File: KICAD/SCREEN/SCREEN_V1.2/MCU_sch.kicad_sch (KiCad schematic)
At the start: 57 parts, among them SW6 SW_SPDT, SW9 SW_SPDT, U1 BD80FC0WEFJ, U12 AMS1117-3.3, U13 AMS1117-3.3, U14 LM2576T-ADJ, U6 ADP2108AUJ-1.8, U9 AMS1117-3.3

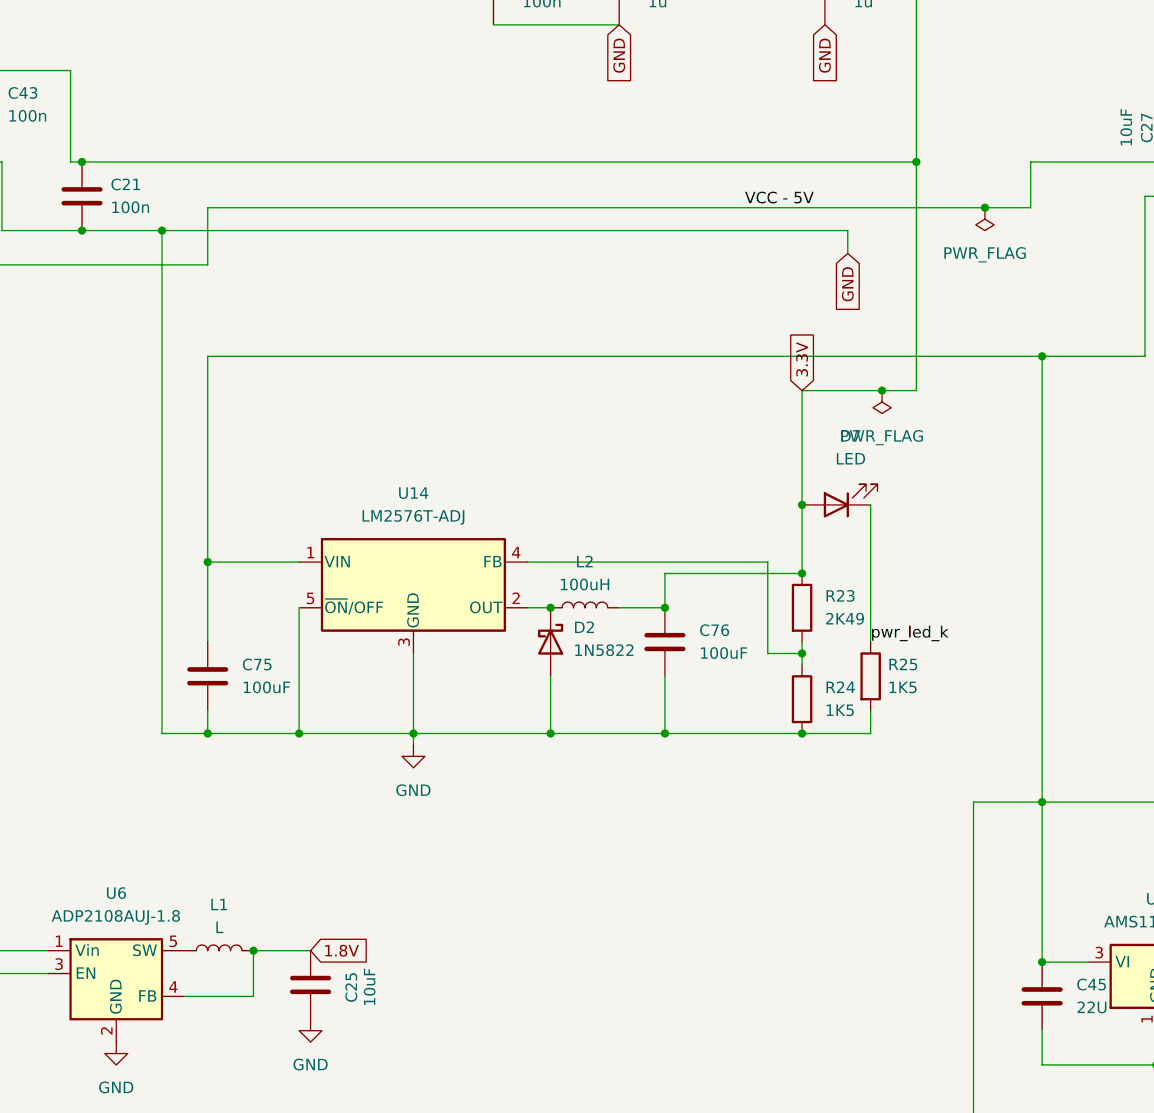
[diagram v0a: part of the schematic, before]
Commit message: .
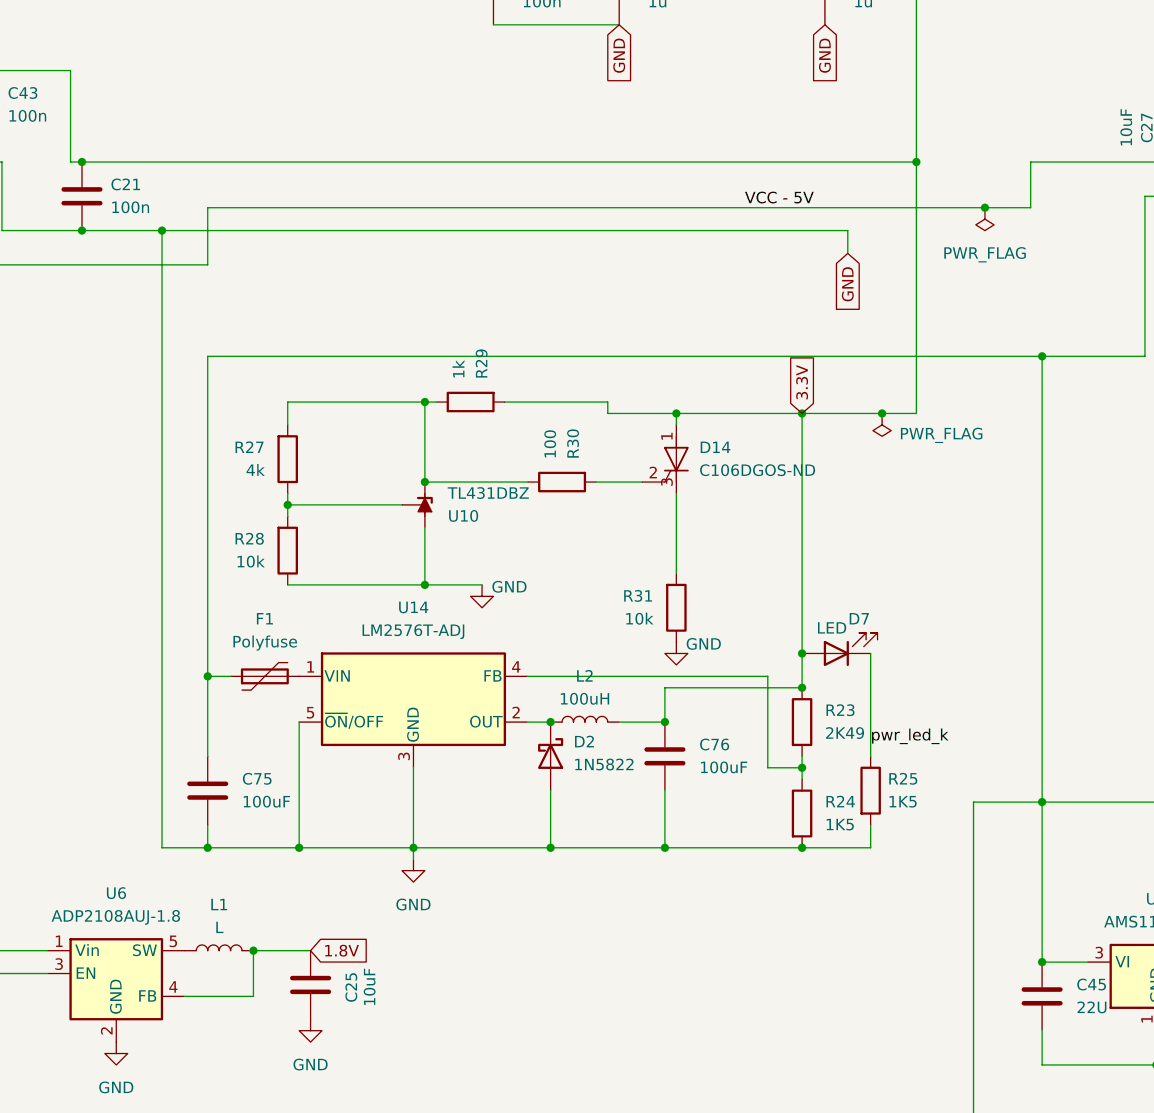
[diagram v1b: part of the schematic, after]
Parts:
- added D14: C106DGOS-ND, Package_SIP:SIP3_11.6x8.5mm, symbol Device:Q_SCR_AGK
- added F1: Polyfuse, Fuse:Fuse_1206_3216Metric, symbol Device:Polyfuse
- added R27: 4k, Resistor_SMD:R_0402_1005Metric, symbol Device:R
- added R28, R31: 10k, Resistor_SMD:R_0402_1005Metric, symbol Device:R
- added R29: 1k, Resistor_SMD:R_0402_1005Metric, symbol Device:R
- added R30: 100, Resistor_SMD:R_0402_1005Metric, symbol Device:R
- added U10: TL431DBZ, Package_TO_SOT_SMD:SOT-23, symbol Reference_Voltage:TL431DBZ
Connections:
- net +12V: now also F1.1; no longer U14.1 (VIN)
- net 3.3V: now also D14.1 (A), R29.2
- net GND: now also R28.1, R31.1, U10.3 (A)
- new net: R27.2, R29.1, R30.1, U10.1 (K)
- new net: R27.1, R28.2, U10.2 (REF)
- new net: F1.2, U14.1 (VIN)
- new net: D14.3 (K), R31.2
- new net: D14.2 (G), R30.2
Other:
- moved on the sheet: C75, C76, D2, D7, L2, R23, R24, R25, U14
